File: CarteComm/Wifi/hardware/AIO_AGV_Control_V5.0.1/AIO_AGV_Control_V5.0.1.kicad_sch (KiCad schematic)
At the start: 7 parts, among them T14 IRF520, U1 L7806, U2 ESP32-WROOM-32, U3 TDN_5-2411WISM

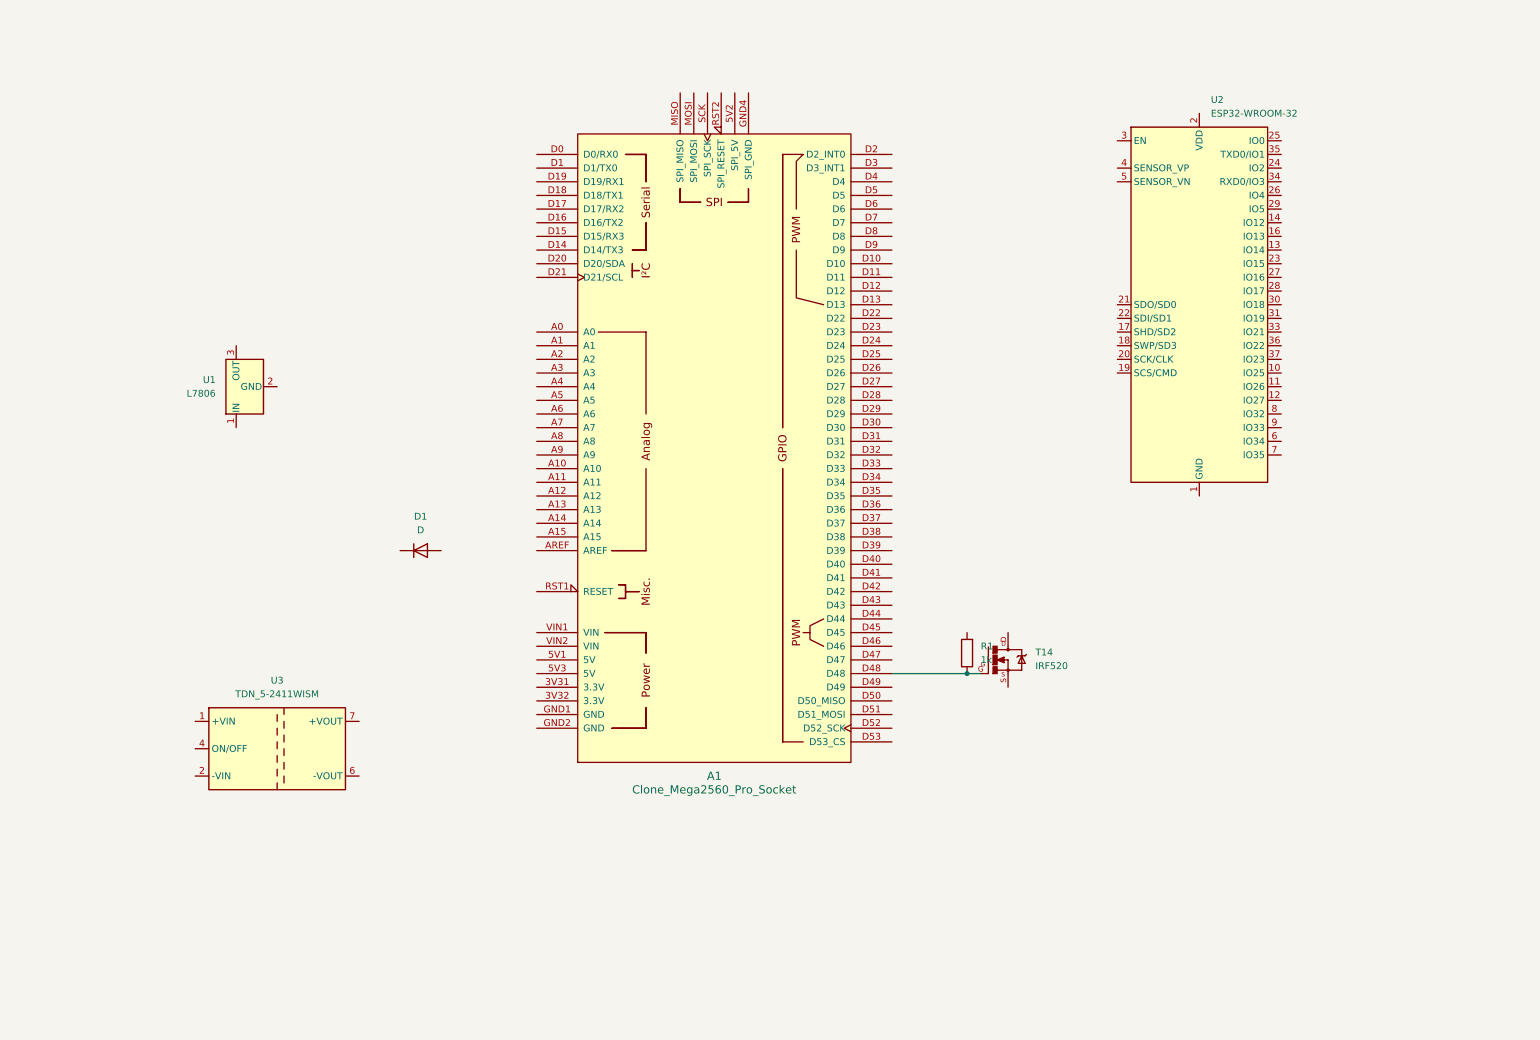
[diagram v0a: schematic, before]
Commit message: KiCad AGV Control 5.0.1
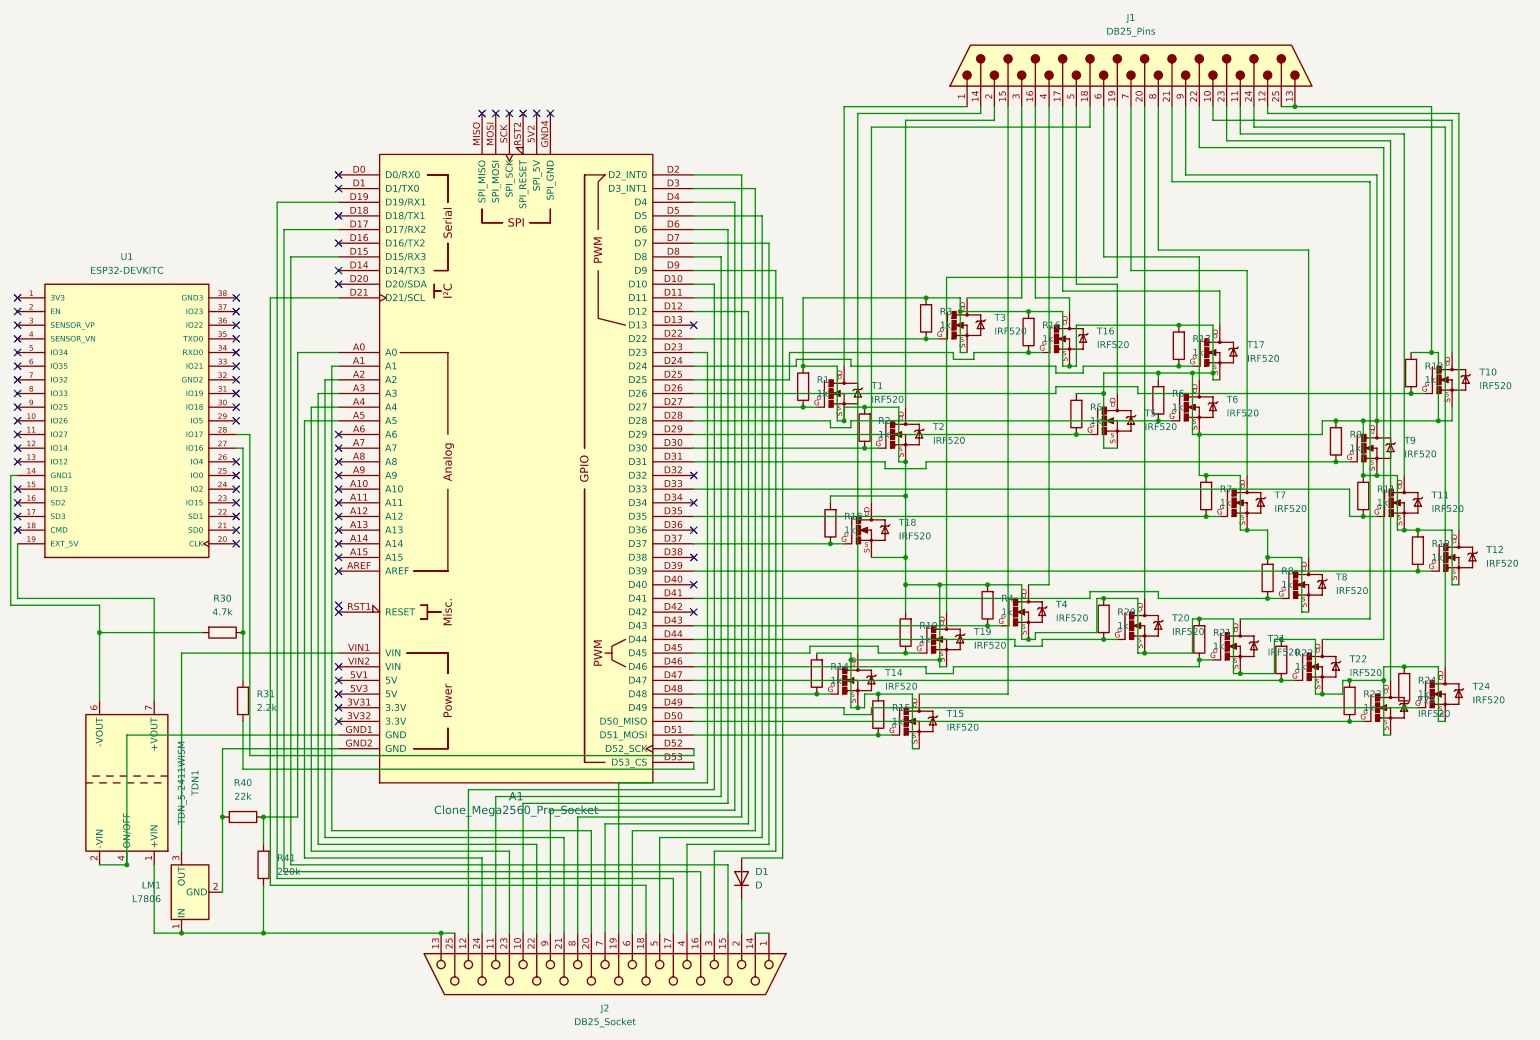
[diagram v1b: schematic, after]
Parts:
- removed U2: ESP32-WROOM-32, RF_Module:ESP32-WROOM-32, symbol RF_Module:ESP32-WROOM-32
- added J1: DB25_Pins, DB25P564CTXLF:AMPHENOL_DB25P564CTXLF, symbol Connector:DB25_Pins
- added J2: DB25_Socket, DB25S564GTLF:AMPHENOL_DB25S564GTLF, symbol Connector:DB25_Socket
- added R1, R10, R11, R12, R15, R16, R17, R18, R19, R2, R20, R21, R22, R23, R24, R3, R4, R5, R6, R7, R8, R9: 1k, Resistor_THT:R_Axial_DIN0411_L9.9mm_D3.6mm_P12.70mm_Horizontal, symbol Device:R
- added R30: 4.7k, Resistor_THT:R_Axial_DIN0411_L9.9mm_D3.6mm_P12.70mm_Horizontal, symbol Device:R
- added R31: 2.2k, Resistor_THT:R_Axial_DIN0411_L9.9mm_D3.6mm_P12.70mm_Horizontal, symbol Device:R
- added R40: 22k, Resistor_THT:R_Axial_DIN0411_L9.9mm_D3.6mm_P12.70mm_Horizontal, symbol Device:R
- added R41: 220k, Resistor_THT:R_Axial_DIN0411_L9.9mm_D3.6mm_P12.70mm_Horizontal, symbol Device:R
- added T1, T10, T11, T12, T15, T16, T17, T18, T19, T2, T20, T21, T22, T23, T24, T3, T4, T5, T6, T7, T8, T9: IRF520, IRF520:TO220BV, symbol IRF520:IRF520
- added U1: ESP32-DEVKITC, ESP32-DEVKITC:MODULE_ESP32-DEVKITC, symbol ESP32-DEVKITC:ESP32-DEVKITC
- LM1: renamed from U1; footprint (none) -> L7806CV:TO255P1020X450X1968-3B
- renumbered R1 to R14, U3 to TDN1
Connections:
- net at LM1.1 (IN): now also TDN1.1 (+VIN), J2.13, J2.25 (P25), R41.1
- net at LM1.2 (GND): now also A1.GND2 (GND), R40.2
- net at LM1.3 (OUT): now also A1.VIN1 (VIN)
- net at T14.D: now also J1.14 (P14)
- net at T14.S: now also R14.2, J1.13, J1.25 (P25), J1.9, R1.2, R10.2, R11.2, R12.2, R15.2, R16.2, R17.2, R18.2, R19.2, R2.2, R20.2, R21.2, R22.2, R23.2, R24.2, R3.2, R4.2, R5.2, R6.2, R7.2, R8.2, R9.2, T1.S, T10.S, T11.S, T12.S, T15.S, T16.S, T17.S, T18.S, T19.S, T2.S, T20.S, T21.S, T22.S, T23.S, T24.S, T3.S, T4.S, T5.S, T6.S, T7.S, T8.S, T9.D, T9.S
- net at D1.1 (K): now also J2.2
- net at D1.2 (A): now also A1.D11
- net at A1.A0: now also R40.1, R41.2
- net at A1.A1: now also J2.20 (P20)
- net at A1.A2: now also J2.21 (P21)
- net at A1.A3: now also J2.22 (P22)
- net at A1.A4: now also J2.23 (P23)
- net at A1.A5: now also J2.24 (P24)
- net at A1.D10: now also J2.12
- net at A1.D12: now also J2.7
- net at A1.D15 (D15/RX3): now also J2.15 (P15)
- net at A1.D17 (D17/RX2): now also J2.16 (P16)
- net at A1.D19 (D19/RX1): now also J2.17 (P17)
- net at A1.D2 (D2_INT0): now also J2.8
- net at A1.D21 (D21/SCL): now also J2.18 (P18)
- net at A1.D22: now also R3.1, T3.G
- net at A1.D23: now also J2.19 (P19)
- net at A1.D24: now also R17.1, T17.G
- net at A1.D25: now also R16.1, T16.G
- net at A1.D26: now also R10.1, T10.G
- net at A1.D27: now also R1.1, T1.G
- net at A1.D28: now also R6.1, T6.G
- net at A1.D29: now also R5.1, T5.G
- net at A1.D3 (D3_INT1): now also J2.6
- net at A1.D30: now also R2.1, T2.G
- net at A1.D31: now also R9.1, T9.G
- net at A1.D33: now also R11.1, T11.G
- net at A1.D35: now also R7.1, T7.G
- net at A1.D37: now also R18.1, T18.G
- net at A1.D39: now also R12.1, T12.G
- net at A1.D4: now also J2.9
- net at A1.D41: now also R8.1, T8.G
- net at A1.D43: now also R4.1, T4.G
- net at A1.D44: now also R20.1, T20.G
- net at A1.D45: now also R19.1, T19.G
- net at A1.D46: now also R21.1, T21.G
- net at A1.D47: now also R22.1, T22.G
- net at A1.D49: now also R24.1, T24.G
- net at A1.D5: now also J2.5
- net at A1.D50 (D50_MISO): now also R23.1, T23.G
- net at A1.D51 (D51_MOSI): now also R15.1, T15.G
- net at A1.D52 (D52_SCK): now also U1.28 (IO17)
- net at A1.D53 (D53_CS): now also R31.1
- net at A1.D6: now also J2.10
- net at A1.D7: now also J2.4
- net at A1.D8: now also J2.11
- net at A1.D9: now also J2.3
- net at A1.GND1 (GND): now also TDN1.2 (-VIN), TDN1.4 (ON/OFF)
- net at TDN1.6 (-VOUT): now also R30.2, U1.14 (GND1)
- net at TDN1.7 (+VOUT): now also U1.19 (EXT_5V)
- new net: J1.6, T6.D
- new net: J1.11, T11.D
- new net: R30.1, R31.2, U1.27 (IO16)
- new net: J1.12, T12.D
- new net: J2.1, J2.14 (P14)
- new net: J1.2, T2.D
- new net: J1.1, T1.D
- new net: J1.10, T10.D
- new net: J1.15 (P15), T15.D
- new net: J1.16 (P16), T16.D
- new net: J1.17 (P17), T17.D
- new net: J1.18 (P18), T18.D
- new net: J1.19 (P19), T19.D
- new net: J1.20 (P20), T20.D
- new net: J1.21 (P21), T21.D
- new net: J1.22 (P22), T22.D
- new net: J1.23 (P23), T23.D
- new net: J1.24 (P24), T24.D
- new net: J1.3, T3.D
- new net: J1.4, T4.D
- new net: J1.5, T5.D
- new net: J1.7, T7.D
- new net: J1.8, T8.D
- no-connect marks 0 -> 71
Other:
- moved on the sheet: A1, D1, LM1, R14, T14, TDN1
